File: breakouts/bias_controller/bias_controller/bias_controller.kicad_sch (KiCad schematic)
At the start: 0 parts

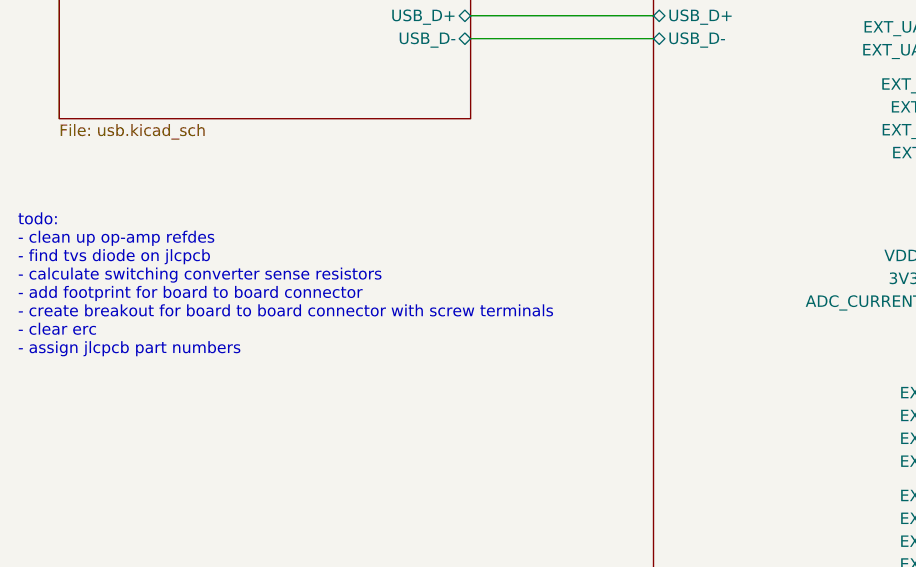
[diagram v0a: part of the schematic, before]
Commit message: added board to board connector
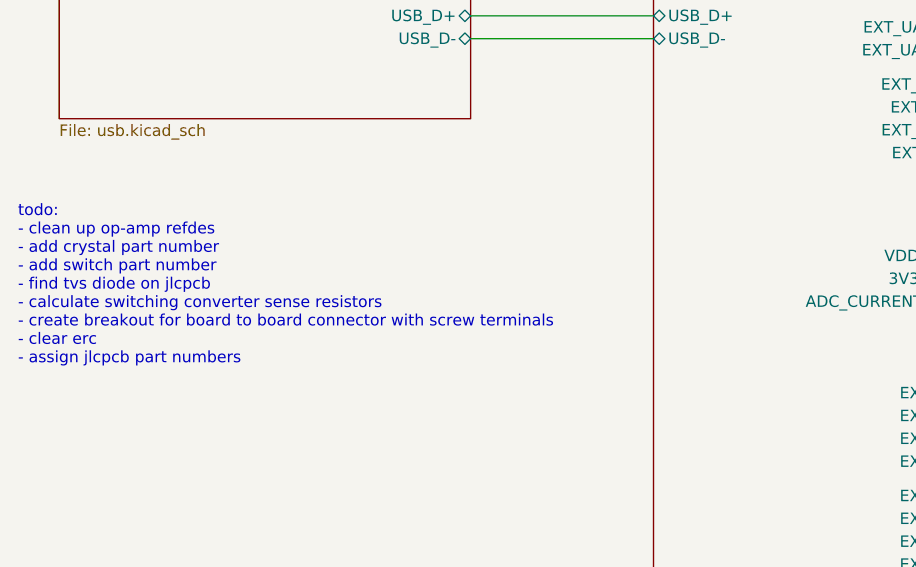
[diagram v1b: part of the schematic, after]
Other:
- note added: "todo: - clean up op-amp refdes - add crystal part number - add switch part number - find tvs diode on jlcpcb - calculate switching converter sense resistors - create breakout for board to board connector with screw terminals - clear erc - assign jlcpcb part numbers"
- note removed: "todo: - clean up op-amp refdes - find tvs diode on jlcpcb - calculate switching converter sense resistors - add footprint for board to board connector - create breakout for board to board connector with screw terminals - clear erc - assign jlcpcb part numbers"
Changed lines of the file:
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@@
 		)
 	)
-	(text "todo:\n- clean up op-amp refdes\n- find tvs diode on jlcpcb\n- calculate switching converter sense resistors\n- add footprint for board to board connector\n- create breakout for board to board connector with screw terminals\n- clear erc\n- assign jlcpcb part numbers"
+	(text "todo:\n- clean up op-amp refdes\n- add crystal part number\n- add switch part number\n- find tvs diode on jlcpcb\n- calculate switching converter sense resistors\n- create breakout for board to board connector with screw terminals\n- clear erc\n- assign jlcpcb part numbers"
 		(exclude_from_sim no)
 		(at 15.748 99.822 0)
